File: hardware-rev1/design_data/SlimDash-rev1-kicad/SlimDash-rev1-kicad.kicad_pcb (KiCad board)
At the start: 2 copper layers, 157.1 x 131.5 mm, 103 parts, among them U1 TLV73333PDBV, U2 RP2040, U3 W25Q128JVS, Y1 Crystal_GND24

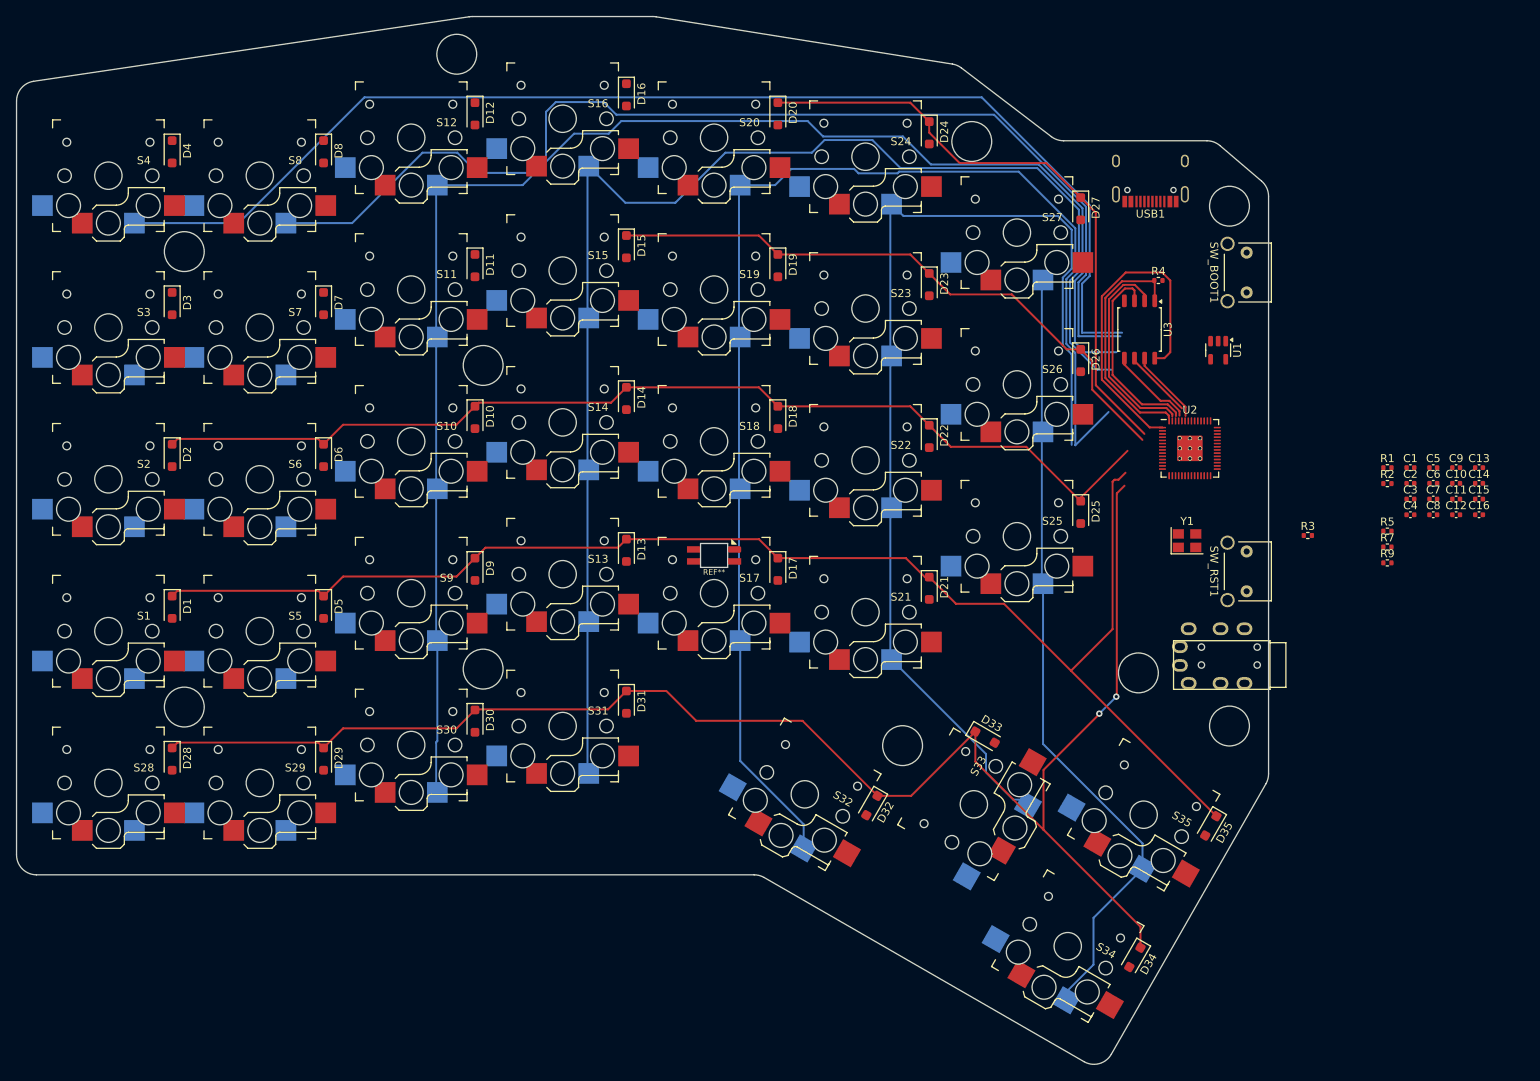
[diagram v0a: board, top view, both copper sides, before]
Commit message: add more components to design data
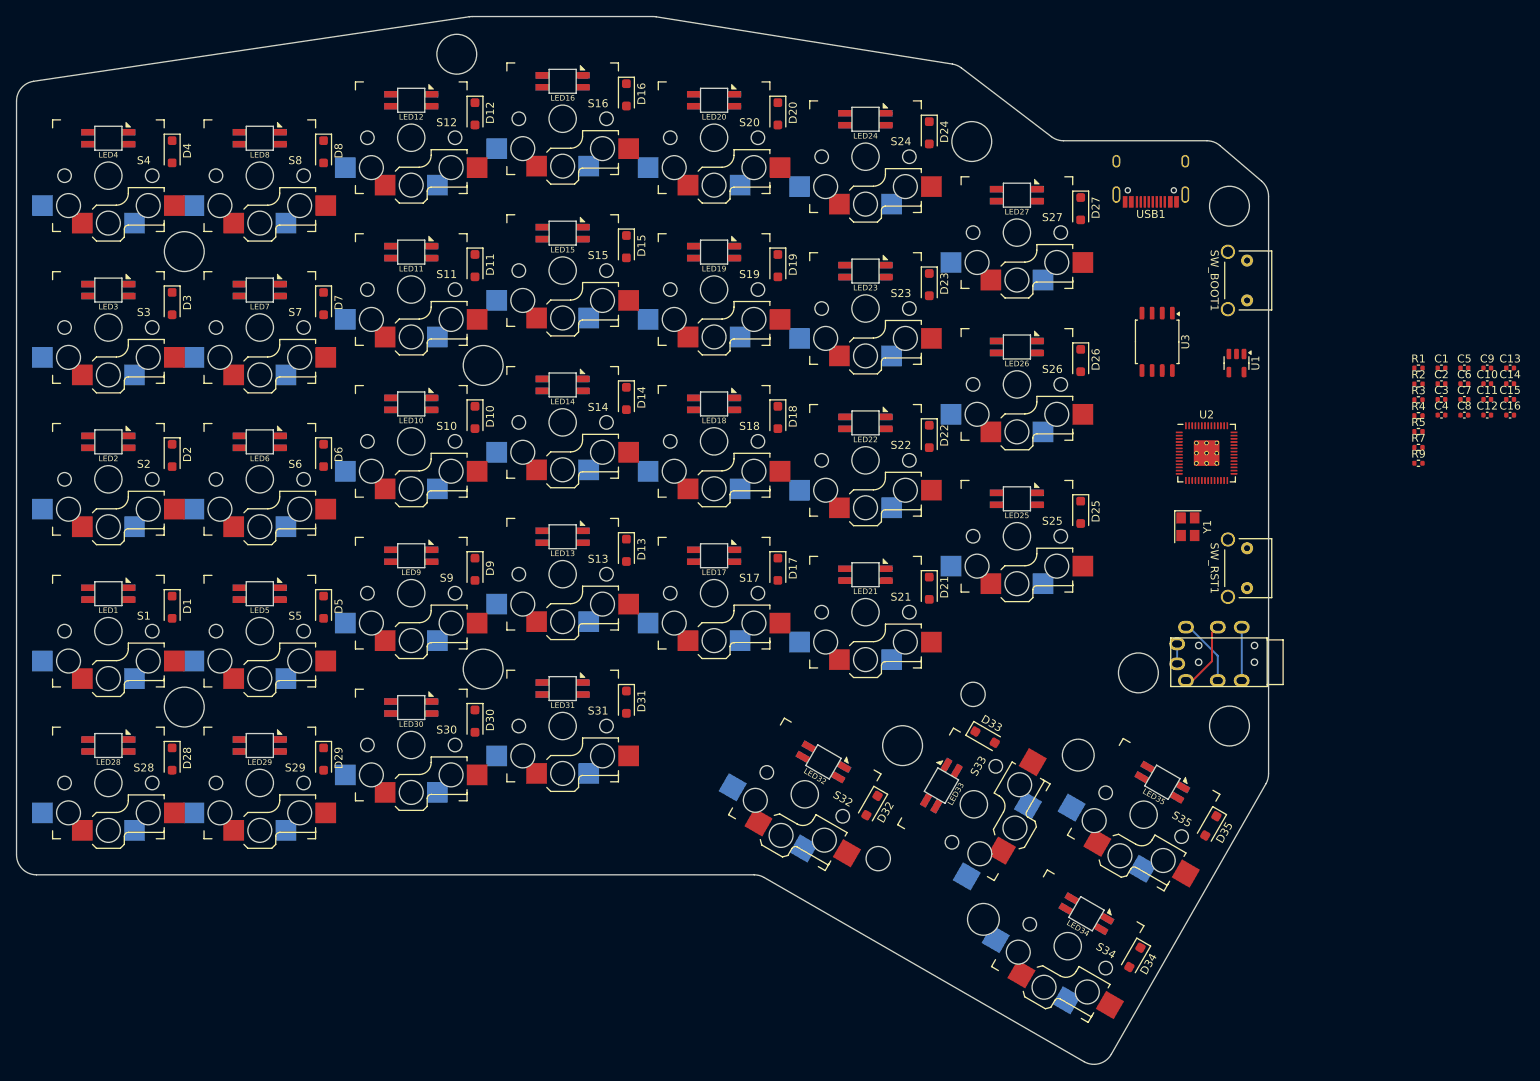
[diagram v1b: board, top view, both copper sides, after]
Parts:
- removed the REF** at (126.0, 90.5)
- removed the REF** at (195.8, 104.2)
- removed the REF** at (195.8, 102.0)
- added J1: AudioJack4, Keebio-Parts:TRRS-PJ-320A, F.Cu at (195.4, 103.9)
- added J2: AudioJack4, Keebio-Parts:TRRS-PJ-320A, B.Cu at (195.4, 101.8)
- added LED1: , mzm_misc:SK6812-MINI-E_Reversible, F.Cu at (50.0, 95.3)
- added LED10: , mzm_misc:SK6812-MINI-E_Reversible, F.Cu at (88.0, 71.5)
- added LED11: , mzm_misc:SK6812-MINI-E_Reversible, F.Cu at (88.0, 52.4)
- added LED12: , mzm_misc:SK6812-MINI-E_Reversible, F.Cu at (88.0, 33.4)
- added LED13: , mzm_misc:SK6812-MINI-E_Reversible, F.Cu at (107.0, 88.2)
- added LED14: , mzm_misc:SK6812-MINI-E_Reversible, F.Cu at (107.0, 69.1)
- added LED15: , mzm_misc:SK6812-MINI-E_Reversible, F.Cu at (107.0, 50.1)
- added LED16: , mzm_misc:SK6812-MINI-E_Reversible, F.Cu at (107.0, 31.0)
- added LED17: , mzm_misc:SK6812-MINI-E_Reversible, F.Cu at (126.0, 90.5)
- added LED18: , mzm_misc:SK6812-MINI-E_Reversible, F.Cu at (126.0, 71.5)
- added LED19: , mzm_misc:SK6812-MINI-E_Reversible, F.Cu at (126.0, 52.4)
- added LED2: , mzm_misc:SK6812-MINI-E_Reversible, F.Cu at (50.0, 76.2)
- added LED20: , mzm_misc:SK6812-MINI-E_Reversible, F.Cu at (126.0, 33.4)
- added LED21: , mzm_misc:SK6812-MINI-E_Reversible, F.Cu at (145.0, 92.9)
- added LED22: , mzm_misc:SK6812-MINI-E_Reversible, F.Cu at (145.0, 73.9)
- added LED23: , mzm_misc:SK6812-MINI-E_Reversible, F.Cu at (145.0, 54.8)
- added LED24: , mzm_misc:SK6812-MINI-E_Reversible, F.Cu at (145.0, 35.8)
- added LED25: , mzm_misc:SK6812-MINI-E_Reversible, F.Cu at (164.0, 83.4)
- added LED26: , mzm_misc:SK6812-MINI-E_Reversible, F.Cu at (164.0, 64.3)
- added LED27: , mzm_misc:SK6812-MINI-E_Reversible, F.Cu at (164.0, 45.3)
- added LED28: , mzm_misc:SK6812-MINI-E_Reversible, F.Cu at (50.0, 114.3)
- added LED29: , mzm_misc:SK6812-MINI-E_Reversible, F.Cu at (69.0, 114.3)
- added LED3: , mzm_misc:SK6812-MINI-E_Reversible, F.Cu at (50.0, 57.2)
- added LED30: , mzm_misc:SK6812-MINI-E_Reversible, F.Cu at (88.0, 109.6)
- added LED31: , mzm_misc:SK6812-MINI-E_Reversible, F.Cu at (107.0, 107.2)
- added LED32: , mzm_misc:SK6812-MINI-E_Reversible, F.Cu at (139.7, 116.4)
- added LED33: , mzm_misc:SK6812-MINI-E_Reversible, F.Cu at (154.5, 119.4)
- added LED34: , mzm_misc:SK6812-MINI-E_Reversible, F.Cu at (172.7, 135.5)
- added LED35: , mzm_misc:SK6812-MINI-E_Reversible, F.Cu at (182.3, 119.0)
- added LED4: , mzm_misc:SK6812-MINI-E_Reversible, F.Cu at (50.0, 38.1)
- added LED5: , mzm_misc:SK6812-MINI-E_Reversible, F.Cu at (69.0, 95.3)
- added LED6: , mzm_misc:SK6812-MINI-E_Reversible, F.Cu at (69.0, 76.2)
- added LED7: , mzm_misc:SK6812-MINI-E_Reversible, F.Cu at (69.0, 57.2)
- added LED8: , mzm_misc:SK6812-MINI-E_Reversible, F.Cu at (69.0, 38.1)
- added LED9: , mzm_misc:SK6812-MINI-E_Reversible, F.Cu at (88.0, 90.5)
- added REF**: Stabilizer_MX_2u, daprice_keyswitches:Stabilizer_MX_2u, F.Cu at (158.6, 121.7)
- moved R4 36.8 mm to (214.4, 73.0)
- moved R3 22.0 mm to (214.4, 71.0)
- moved C1 13.1 mm to (217.3, 67.0)
- moved C13 13.1 mm to (225.9, 67.0)
- moved C14 13.1 mm to (225.9, 69.0)
- moved C15 13.1 mm to (225.9, 70.9)
- moved C16 13.1 mm to (225.9, 72.9)
- moved C2 13.1 mm to (217.3, 69.0)
- moved C3 13.1 mm to (217.3, 70.9)
- moved C4 13.1 mm to (217.3, 72.9)
- moved C5 13.1 mm to (220.1, 67.0)
- moved C6 13.1 mm to (220.1, 69.0)
- moved C7 13.1 mm to (220.1, 70.9)
- moved C8 13.1 mm to (220.1, 72.9)
- moved R1 13.1 mm to (214.4, 67.0)
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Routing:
- net ROW4: track 196.0 -> 0.00 mm, vias 2 -> 0
- net COL2: track 188.5 -> 0.00 mm
- net ROW3: track 176.9 -> 0.00 mm
- net COL3: track 170.8 -> 0.00 mm
- net COL4: track 167.1 -> 0.00 mm
- net COL0: track 153.4 -> 0.00 mm
- net COL1: track 139.4 -> 0.00 mm
- net COL5: track 136.8 -> 0.00 mm
- net ROW2: track 132.2 -> 0.00 mm
- net COL6: track 99.7 -> 0.00 mm
- net ROW1: track 77.5 -> 0.00 mm
- net ROW0: track 76.7 -> 0.00 mm
- net +3V3: track 42.0 -> 2.51 mm
- net QSPI_SS: track 29.9 -> 0.00 mm
- net QSPI_SD1: track 26.4 -> 0.00 mm
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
